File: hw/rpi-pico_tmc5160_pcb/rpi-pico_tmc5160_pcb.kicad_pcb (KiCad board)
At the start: 2 copper layers, 99 x 87 mm, 9 parts, among them J1 Conn_01x04, J2 Conn_01x03, J3 Conn_01x04, J4 Conn_01x04, J5 Conn_01x04, U1 Pico

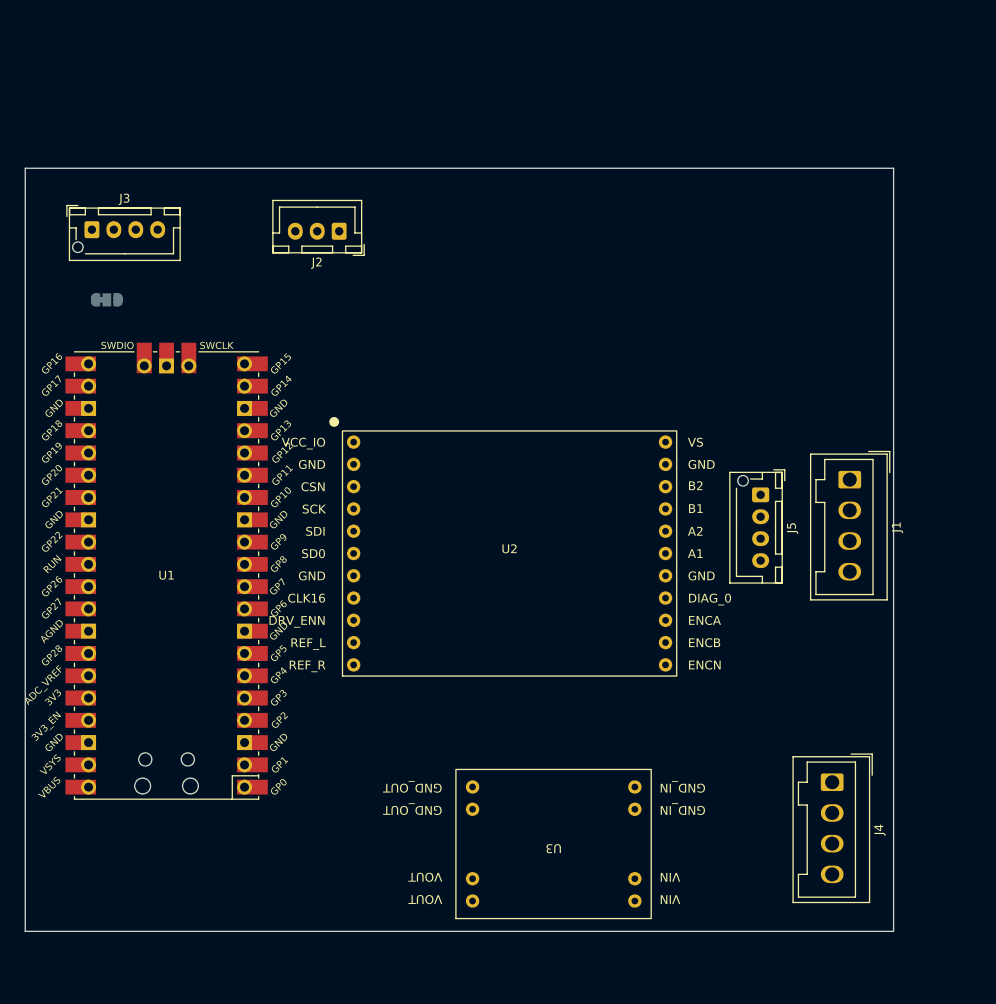
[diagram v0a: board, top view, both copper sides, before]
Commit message: first PCB layout
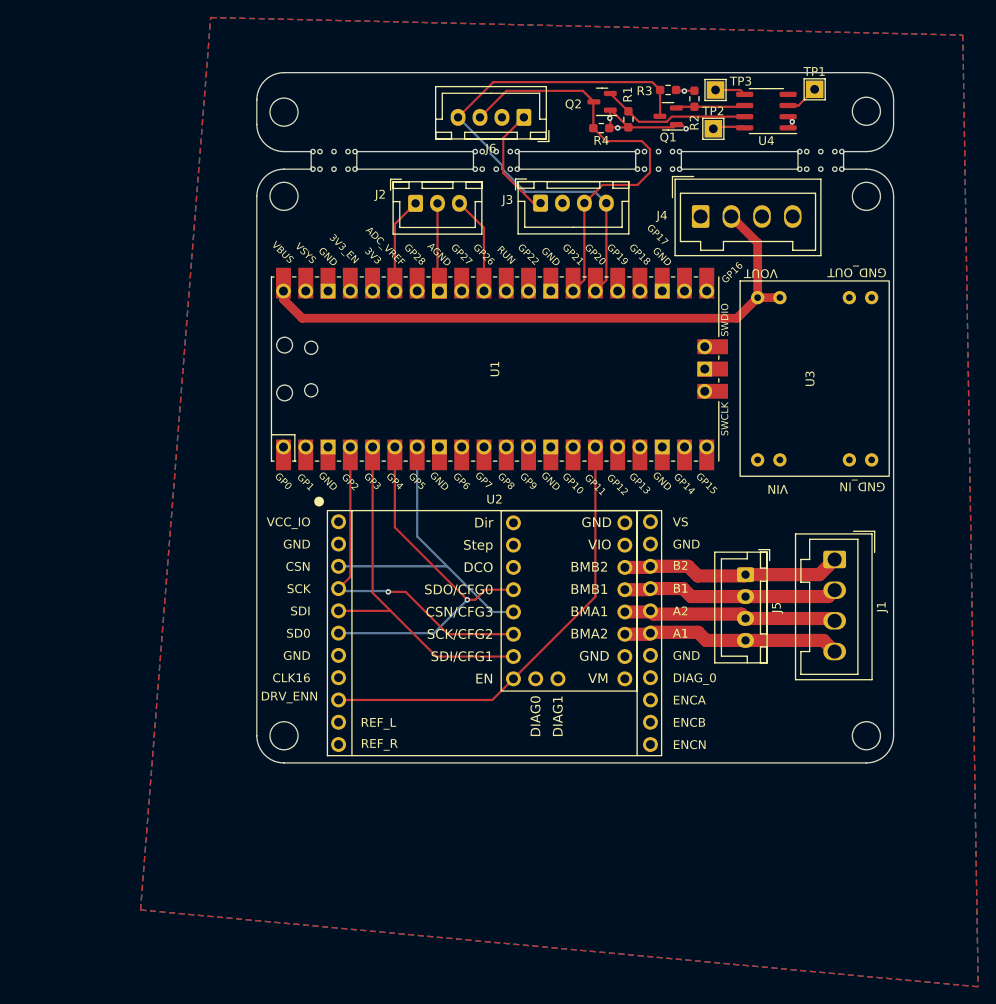
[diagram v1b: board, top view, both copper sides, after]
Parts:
- removed JP1: Jumper_3_Bridged12, Jumper:SolderJumper-3_P1.3mm_Bridged12_RoundedPad1.0x1.5mm
- added H1: MountingHole, MountingHole:MountingHole_3.2mm_M3_ISO7380, F.Cu at (96.5, 39.2)
- added H2: MountingHole, MountingHole:MountingHole_3.2mm_M3_ISO7380, F.Cu at (162.9, 39.2)
- added H3: MountingHole, MountingHole:MountingHole_3.2mm_M3_ISO7380, F.Cu at (162.9, 100.7)
- added H4: MountingHole, MountingHole:MountingHole_3.2mm_M3_ISO7380, F.Cu at (96.5, 100.7)
- added H5: MountingHole, MountingHole:MountingHole_3.2mm_M3_ISO7380, F.Cu at (96.5, 29.6)
- added H6: MountingHole, MountingHole:MountingHole_3.2mm_M3_ISO7380, F.Cu at (162.9, 29.5)
- added J6: Conn_01x04, Connector_JST:JST_XH_B4B-XH-A_1x04_P2.50mm_Vertical, F.Cu at (123.8, 30.2)
- added N1: Housing, project:Mousebite, F.Cu at (102.2, 35.1)
- added N2: Housing, project:Mousebite, F.Cu at (120.7, 35.1)
- added N3: Housing, project:Mousebite, F.Cu at (139.2, 35.1)
- added N4: Housing, project:Mousebite, F.Cu at (157.7, 35.1)
- added Q1: 2N7002, Package_TO_SOT_SMD:SOT-23, F.Cu at (140.3, 30.1)
- added Q2: 2N7002, Package_TO_SOT_SMD:SOT-23, F.Cu at (132.8, 28.4)
- added R1: 4k7, Resistor_SMD:R_0603_1608Metric_Pad0.98x0.95mm_HandSolder, F.Cu at (135.8, 30.4)
- added R2: 4k7, Resistor_SMD:R_0603_1608Metric_Pad0.98x0.95mm_HandSolder, F.Cu at (143.3, 28.1)
- added R3: 4k7, Resistor_SMD:R_0603_1608Metric_Pad0.98x0.95mm_HandSolder, F.Cu at (140.3, 27.1)
- added R4: 4k7, Resistor_SMD:R_0603_1608Metric_Pad0.98x0.95mm_HandSolder, F.Cu at (132.7, 31.4)
- added TP1: TestPoint, TestPoint:TestPoint_THTPad_2.0x2.0mm_Drill1.0mm, F.Cu at (157.0, 27.0)
- added TP2: TestPoint, TestPoint:TestPoint_THTPad_2.0x2.0mm_Drill1.0mm, F.Cu at (145.4, 31.5)
- added TP3: TestPoint, TestPoint:TestPoint_THTPad_2.0x2.0mm_Drill1.0mm, F.Cu at (145.7, 27.1)
- added U4: AS5600, Package_SO:SOIC-8_3.9x4.9mm_P1.27mm, F.Cu at (151.5, 29.5)
- J3, J5: footprint Connector_JST:JST_XH_B4B-XH-AM_1x04_P2.50mm_Vertical -> Connector_JST:JST_XH_B4B-XH-A_1x04_P2.50mm_Vertical
- U3: value ~ -> MP1584
- moved J4 66.2 mm to (144.0, 41.5), turned to 0 degrees
- moved U3 60.8 mm to (157.0, 60.0), turned to 90 degrees
- moved J3 51.2 mm to (125.8, 40.0)
- moved U1 44.2 mm to (120.6, 58.9), turned to 90 degrees
- moved J2 9.27 mm to (111.5, 40.0), turned to 0 degrees
- moved J1 9.26 mm to (159.3, 80.6)
- moved J5 9.26 mm to (149.1, 82.3)
- moved U2 9.24 mm to (120.5, 89.0)
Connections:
- J2 pad 1: /A0 -> VDDA
- J2 pad 2: VDDA -> GNDA
- J2 pad 3: GNDA -> /A0
- J3 pad 1: /VDD_I2C -> +3V3
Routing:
- net +5V: track 0.00 -> 69.9 mm
- net /SDA_0: track 0.00 -> 60.1 mm
- net /DRV_ENN: track 0.00 -> 51.2 mm
- net /SCL_0: track 0.00 -> 47.4 mm
- net /SDO: track 0.00 -> 42.8 mm, vias 0 -> 1
- net /SDI: track 0.00 -> 41.6 mm
- net /SCK: track 0.00 -> 38.8 mm, vias 0 -> 1
- net /CSN: track 0.00 -> 37.1 mm
- net +3V3: track 0.00 -> 30.9 mm, vias 0 -> 5
- net /M_B2: track 0.00 -> 25.2 mm
- net /M_A1: track 0.00 -> 24.9 mm
- net /M_B1: track 0.00 -> 24.7 mm
- net /M_A2: track 0.00 -> 24.4 mm
- net Net-(Q2-S): track 0.00 -> 16.9 mm
- net /A0: track 0.00 -> 11.2 mm
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- added copper zone on In2.Cu, net +24V
- added copper zone on In1.Cu, net +3V3
- added copper zone on B.Cu, net GND
- added copper zone on F.Cu, net GND
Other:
- board size 99 x 87 mm -> 72.6 x 78.7 mm
- copper layers 2 -> 4
- board text added: "RPi-Pico_TMC5160 Rev. - Author: fitsnot"
